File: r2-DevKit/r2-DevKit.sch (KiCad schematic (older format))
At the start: 29 parts, among them CON1 USB-MICRO-B, J1 CONN_01X05, J10 Battery SW, J11 OPTS, J2 CONN_01X08, J3 CONN_01X14, J4 CONN_01X02, J5 CONN_01X08, J6 CONN_01X14, J7 Li-Po, J8 JTAG, J9 CONN_02X15, P1 Compute Socket, P2 Sensor Socket, P3 CONN_01X01, P4 CONN_01X01, SW3 Pin_0, SW4 CHIP_PU, U1 EMIF02-USB03F2

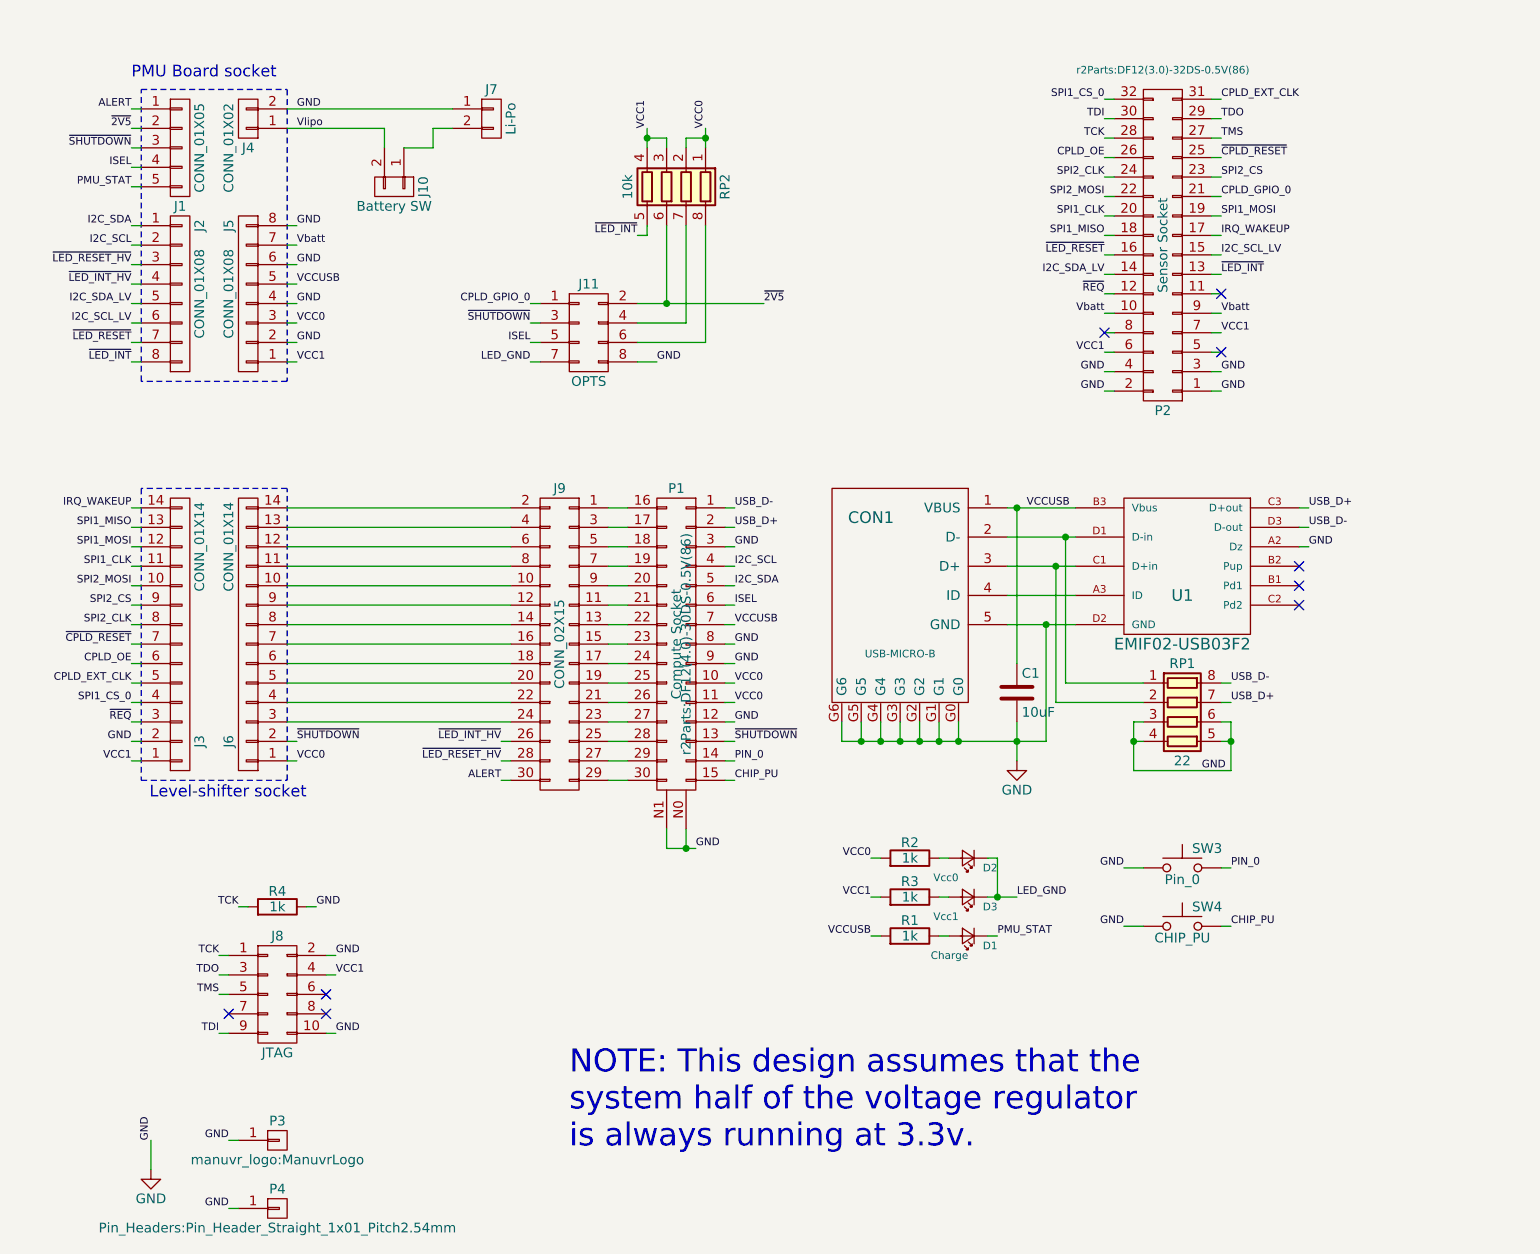
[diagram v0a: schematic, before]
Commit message: Adding BOM info.
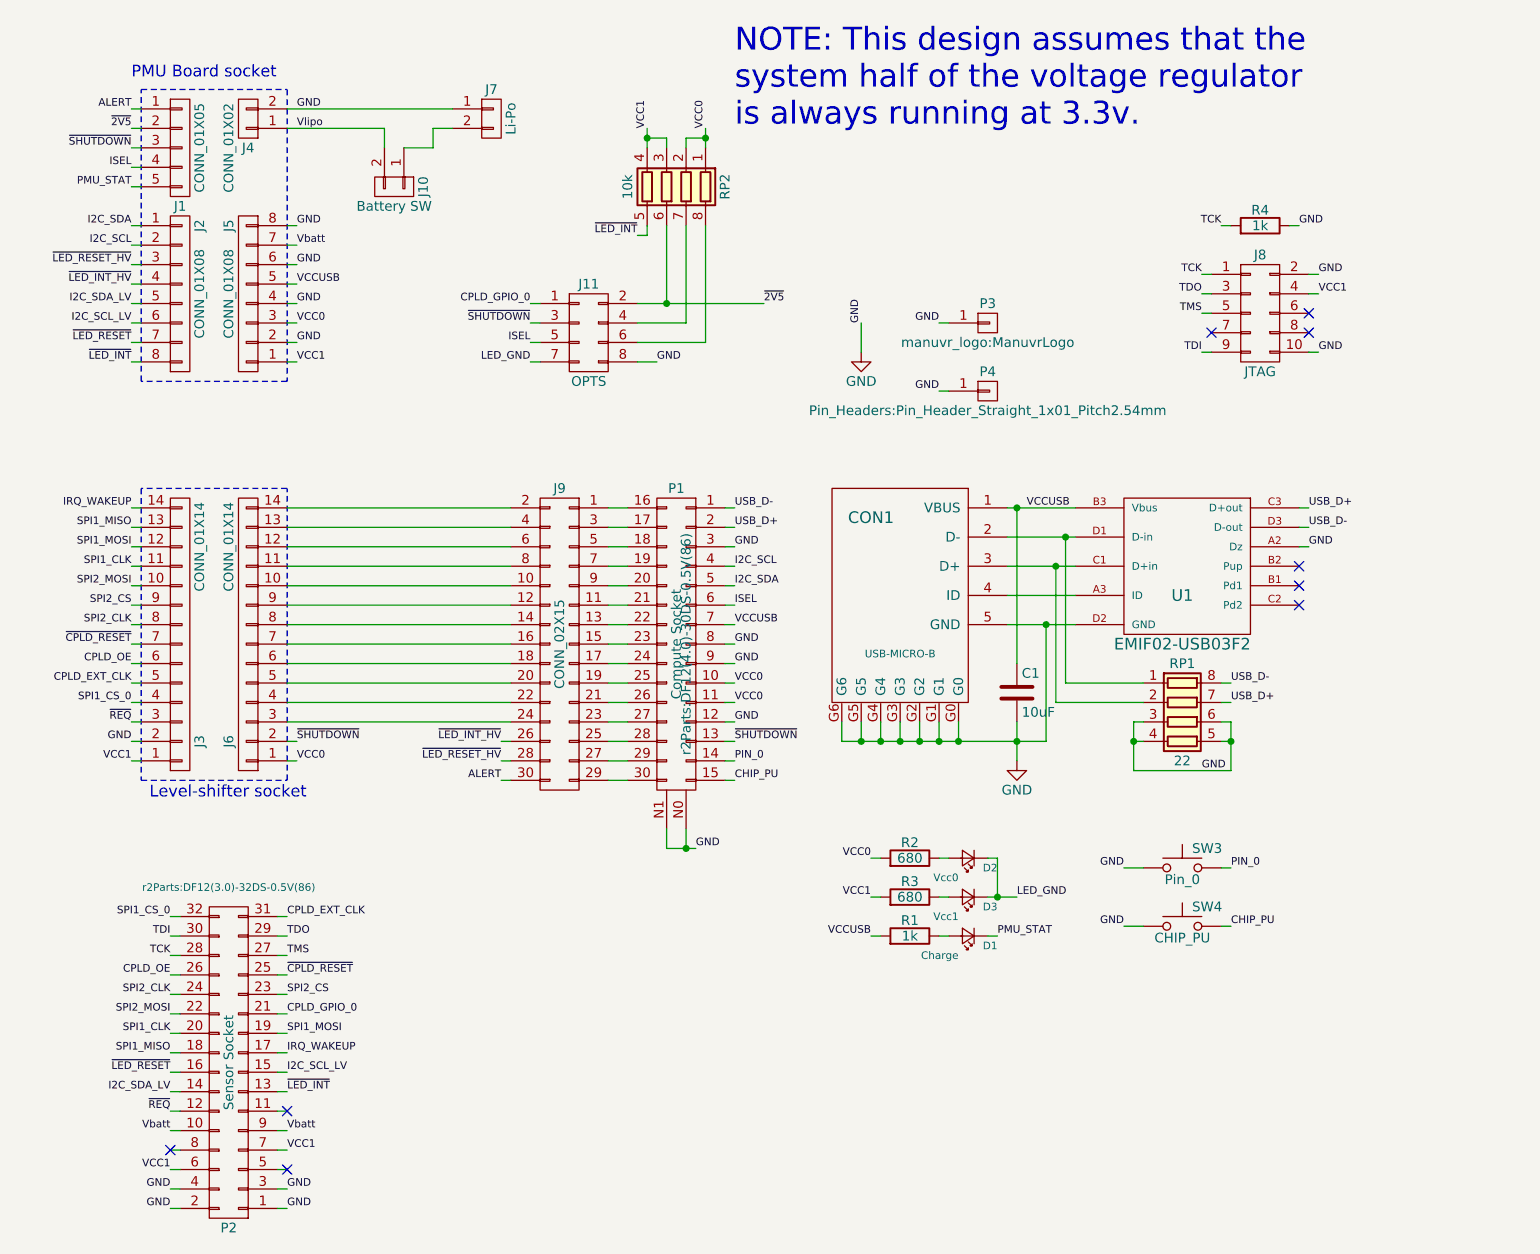
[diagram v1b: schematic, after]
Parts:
- D1, D2, D3: footprint Resistors_SMD:R_0402_NoSilk -> Diodes_SMD:D_0603; Digikey_Number LNJ347W83RACT-ND -> 732-4971-1-ND; Manu_Name Panasonic Electronic Components -> Wurth Electronics Inc.; Manu_Number LNJ347W83RA -> 150060GS75000
- J7: DigikeyNum 455-1749-6-ND -> (none); Digikey_Number (none) -> 455-1749-6-ND; ManuName JST Sales America Inc. -> (none); ManuNum S2B-PH-SM4-TB(LF)(SN) -> (none); Manu_Name (none) -> JST Sales America Inc.; Manu_Number (none) -> S2B-PH-SM4-TB(LF)(SN)
- R1, R4: Digikey_Number P1.00KLCT-ND -> 311-1.0KJRCT-ND; Manu_Name Panasonic Electronic Components -> Yageo; Manu_Number ERJ-2RKF1001X -> RC0402JR-071KL
- R2, R3: value 1k -> 680; Digikey_Number P1.00KLCT-ND -> 311-680JRCT-ND; Manu_Name Panasonic Electronic Components -> Yageo; Manu_Number ERJ-2RKF1001X -> RC0402JR-07680RL
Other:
- moved on the sheet: J8, P2, P3, P4
